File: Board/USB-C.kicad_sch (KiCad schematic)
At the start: 2 parts, among them J2 USB_C_Receptacle_USB2.0_16P, U6 INA226

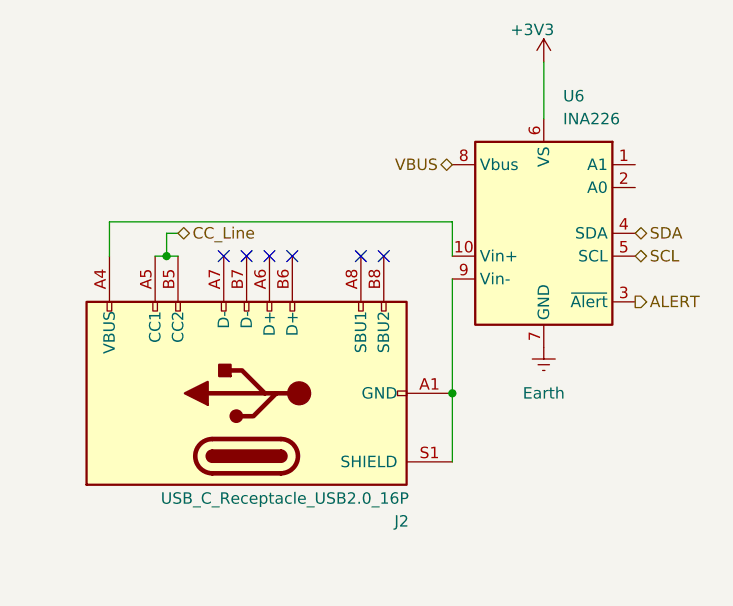
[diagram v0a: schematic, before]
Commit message: Finished Schematic
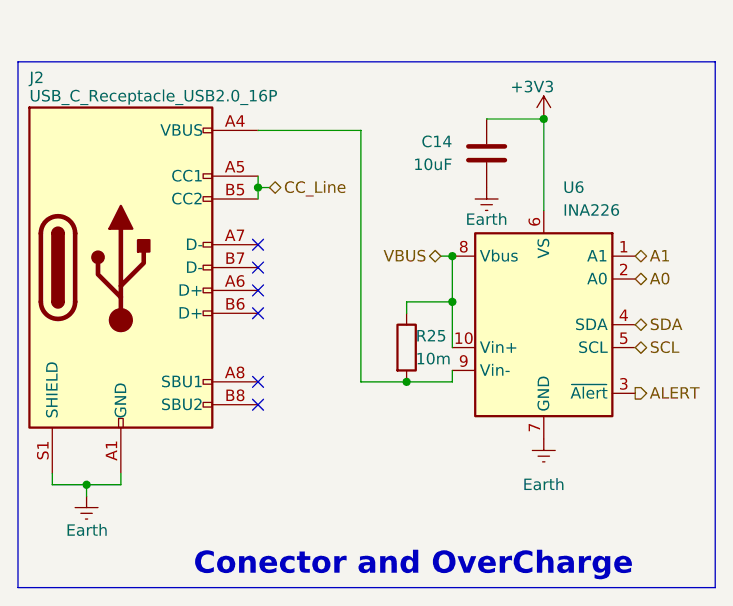
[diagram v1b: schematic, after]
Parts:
- added C14: 10uF, Capacitor_SMD:C_0603_1608Metric, symbol Device:C
- added R25: 10m, Resistor_SMD:R_0603_1608Metric, symbol Device:R
- J2: footprint (none) -> Library:CONN_USB4145-03-0230-C_GCT
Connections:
- net +3V3: now also C14.1
- net Earth: now also J2.A1 (GND), J2.A12 (GND), J2.B1 (GND), J2.B12 (GND), J2.S1 (SHIELD), C14.2
- net VBUS: now also U6.10 (Vin+), R25.1
- net A1: now reaches U6.1 (A1)
- net at J2.A4 (VBUS), J2.A9 (VBUS), J2.B4 (VBUS)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: now also U6.9 (Vin-), R25.2; no longer U6.10 (Vin+)
- net A0: now reaches U6.2 (A0)
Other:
- note added: "Conector and OverCharge"
- moved on the sheet: J2, U6
